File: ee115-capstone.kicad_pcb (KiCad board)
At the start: 4 copper layers, 191 parts, among them J1 2171790001, J2 9V_BATTERY, J3 Conn_01x04_Pin, J5 Conn_01x03_Pin, J6 Conn_02x02_Odd_Even, Q1 PMOS, Q2 NMOS, Q3 NPN, Q4 AO3400A, Q5 AO3400A, Q6 NMOS, Q7 PNP, Q8 NPN, SW1 SW_Push, SW2 SW_Push, SW3 SW_Push, U1 OPA2140AIDR, U10 SN74LVC1G02DCKR (NOR), U11 SN74LVC1G02DCKR (NOR), U12 ALD1107PBL, U13 LD39150DT33-R, U14 SL78L05, U15 300P14-U, U16 OPA705PA, U17 MIC4605-2YM-TR, U18 OPA705PA, U19 OPA705PA, U2 CD4052BPWR, U20 AD8038, U21 MCP6571T-E/OT, U3 LM393DR, U4 ADG601BRMZ-REEL7, U5 ESP32-C3-WROOM-02-N4, U6 AP2112K-3.3, U7 MCP601T-E_OT, U8 MCP6571T-E/OT, U9 MCP6571T-E/OT

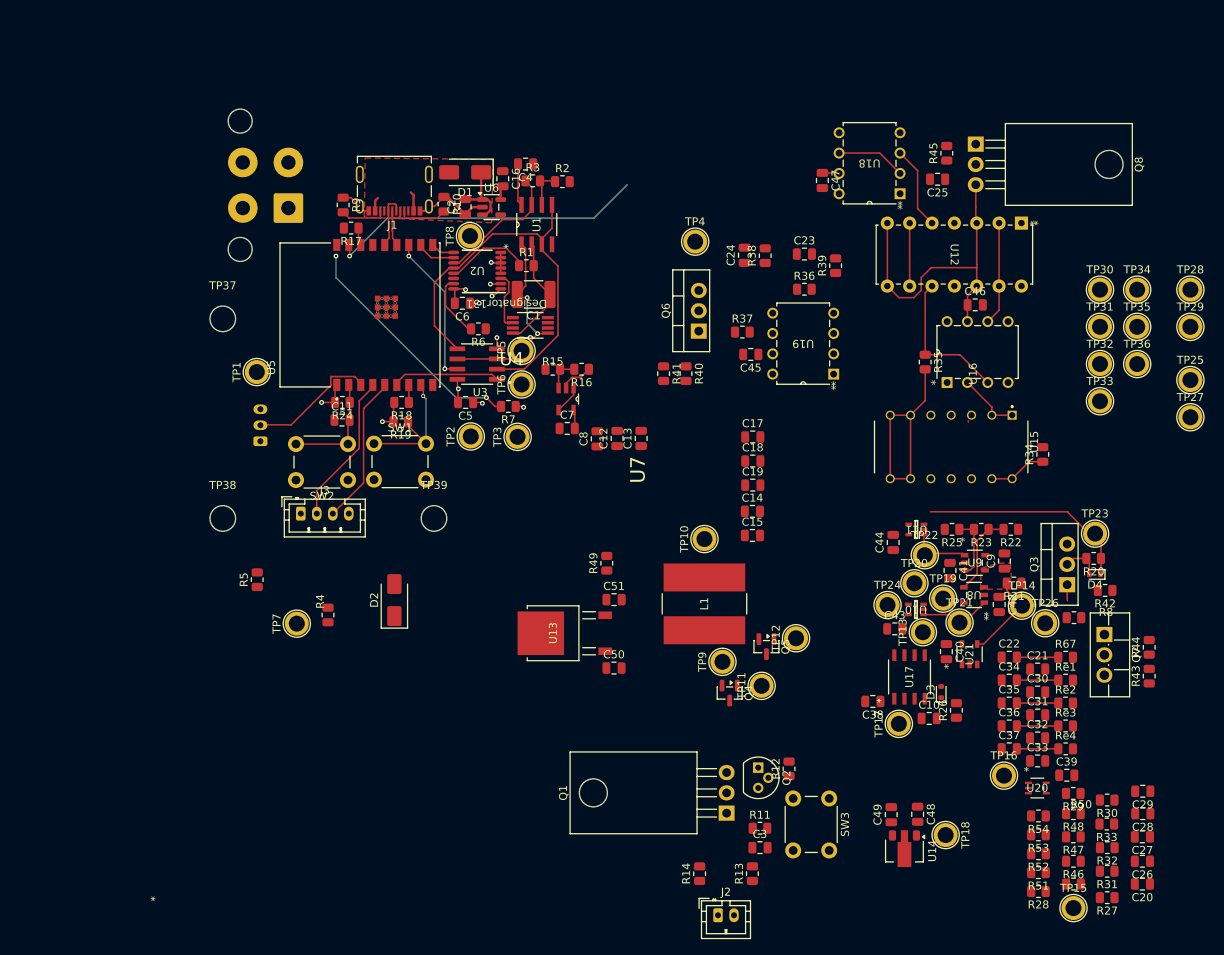
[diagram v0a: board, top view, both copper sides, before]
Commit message: init pcb
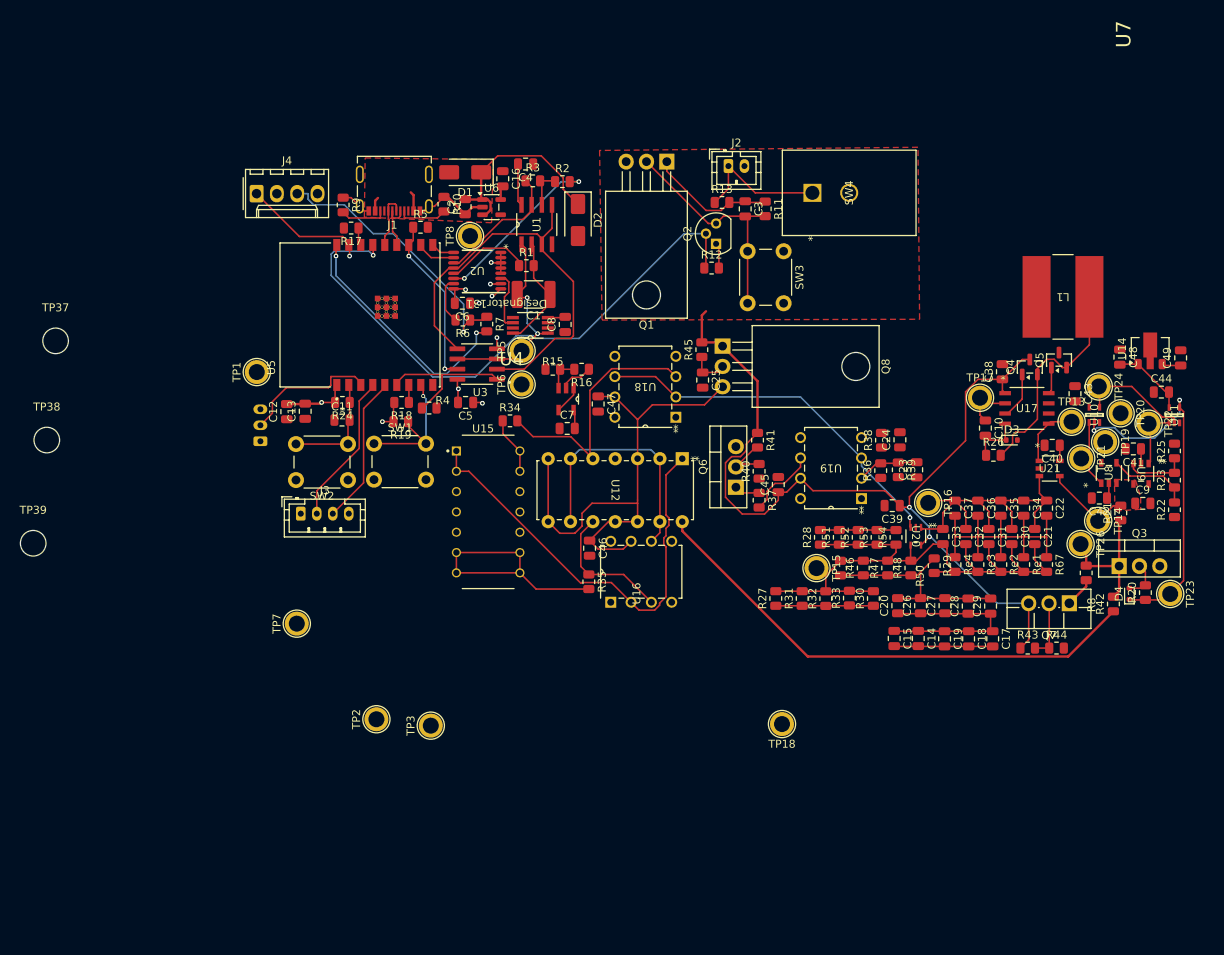
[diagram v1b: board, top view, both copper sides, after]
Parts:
- removed C50, C51: C, Capacitor_SMD:C_0805_2012Metric
- removed J6: Conn_02x02_Odd_Even, Connector_Molex:Molex_Mega-Fit_76829-0004_2x02_P5.70mm_Vertical
- removed R14, R49: 0, Resistor_SMD:R_0805_2012Metric
- removed TP10, TP11, TP12, TP25, TP27, TP28, TP29, TP30, TP31, TP32, TP33, TP34, TP35, TP36, TP4, TP9: TestPoint, TestPoint:TestPoint_Plated_Hole_D2.0mm
- removed U13: LD39150DT33-R, footprints_pretty:SOT_0DT33-R_STM
- added J4: Conn_01x04_Pin, Connector_Molex:Molex_KK-254_AE-6410-04A_1x04_P2.54mm_Vertical, F.Cu at (60.6, 100.5)
- added SW4: GF-123-0054, footprints:SW2_GF-123-0054_CWI, F.Cu at (130.1, 100.4)
- moved J2 93.7 mm to (119.6, 97.0)
- moved R13 84.0 mm to (118.8, 101.6), turned to 0 degrees
- moved Q1 81.8 mm to (111.9, 96.5), turned to 180 degrees
- moved C3 79.9 mm to (121.7, 102.4), turned to -90 degrees
- moved R11 77.4 mm to (124.2, 102.4), turned to -90 degrees
- moved U14 69.9 mm to (172.3, 119.9), turned to 90 degrees
- moved SW3 68.6 mm to (126.5, 107.7)
- moved C49 67.6 mm to (176.1, 121.0)
- moved R34 66.7 mm to (92.3, 128.9), turned to 0 degrees
- moved Q2 65.7 mm to (118.1, 106.8), turned to 90 degrees
- moved R12 63.3 mm to (117.5, 109.8), turned to 0 degrees
- moved C48 62.5 mm to (168.5, 120.9)
- moved L1 59.0 mm to (161.4, 113.4), turned to 180 degrees
- moved U15 58.4 mm to (89.6, 140.3), turned to 0 degrees
- moved C46 57.0 mm to (102.2, 144.8), turned to -90 degrees
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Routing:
- net +9V: track 0.00 -> 134.2 mm, vias 0 -> 2
- net Net-(U20--): track 0.00 -> 78.8 mm
- net /POWER_LATCH: track 0.00 -> 73.8 mm, vias 0 -> 1
- net /Buck Converter/I_PTAT: track 0.00 -> 63.9 mm
- net /bandgap/minus: track 7.89 -> 55.5 mm
- net /Buck Converter/error: track 0.00 -> 41.9 mm
- net +3.5V: track 0.00 -> 38.4 mm
- net GND: track 26.8 -> 64.9 mm
- net /Buck Converter/bg_volt: track 8.67 -> 46.3 mm, vias 0 -> 1
- net /Thermopile: track 1.03 -> 34.5 mm
- net Net-(Q1-G): track 0.00 -> 29.4 mm
- net /Buck Converter/switch_node: track 0.00 -> 28.0 mm
- net Net-(C20-Pad2): track 0.00 -> 27.5 mm
- net /bandgap/pwr_bus: track 41.7 -> 66.4 mm
- net /Thermistor: track 39.8 -> 15.8 mm
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- added copper zone on F.Cu, net +9V
- added copper zone on In1.Cu, net GND
